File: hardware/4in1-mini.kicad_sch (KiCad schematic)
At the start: 23 parts, among them J1 SM08B-SRSS-TB, U1 TLV76733DRVR, U12 INA186A3IDCKR, U13 LMR54406DBVR, U5 FTC160808S4R7MBCA

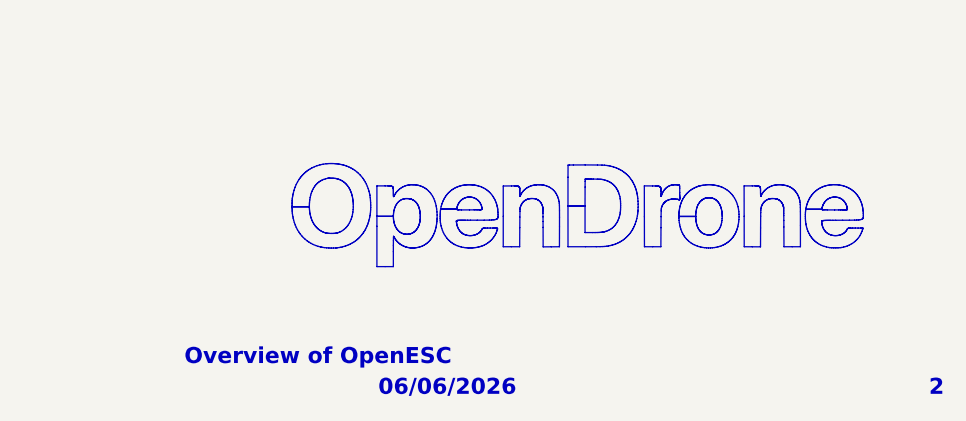
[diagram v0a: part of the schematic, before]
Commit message: SFT naming update
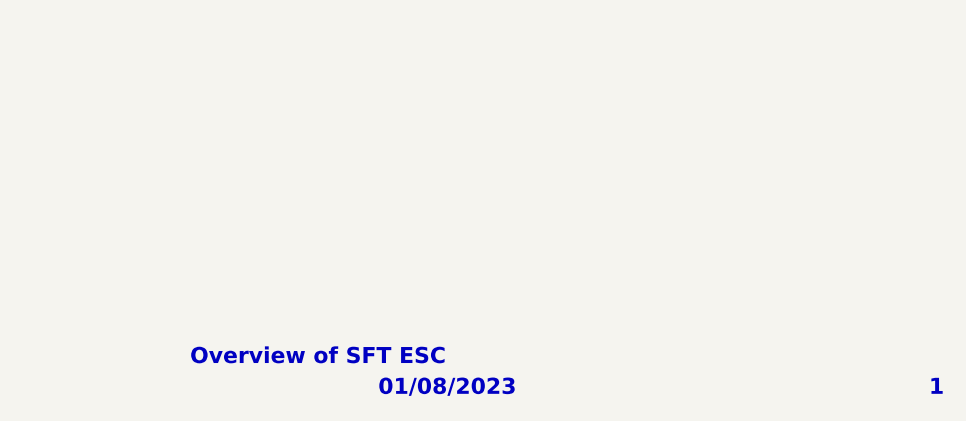
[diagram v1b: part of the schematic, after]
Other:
- note added: "01/08/2023"
- note added: "1"
- note added: "Overview of SFT ESC"
- note removed: "06/06/2026"
- note removed: "2"
- note removed: "Overview of OpenESC"
